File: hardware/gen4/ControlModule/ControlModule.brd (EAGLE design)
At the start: 29.9 x 59.3 mm, 39 parts, among them IC1 XMEGA16A4A

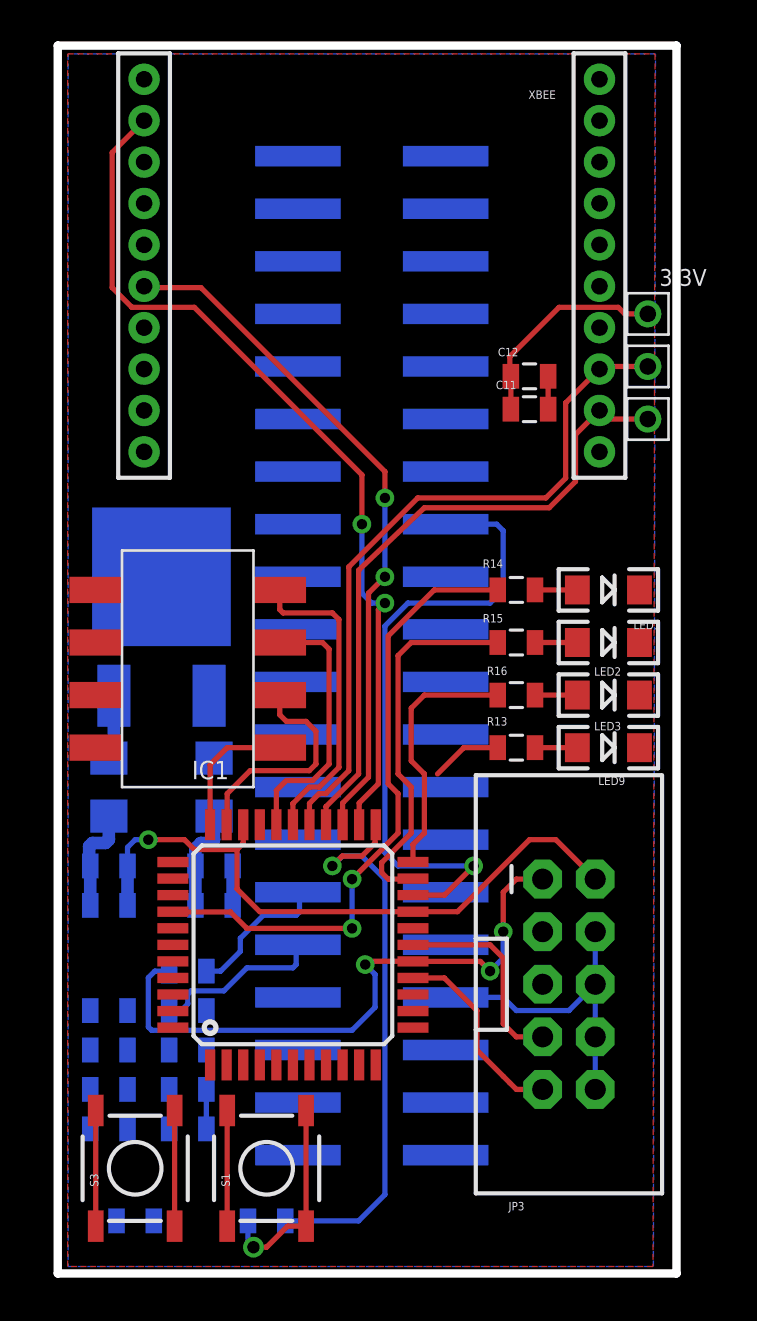
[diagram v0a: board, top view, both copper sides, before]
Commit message: routing fun!
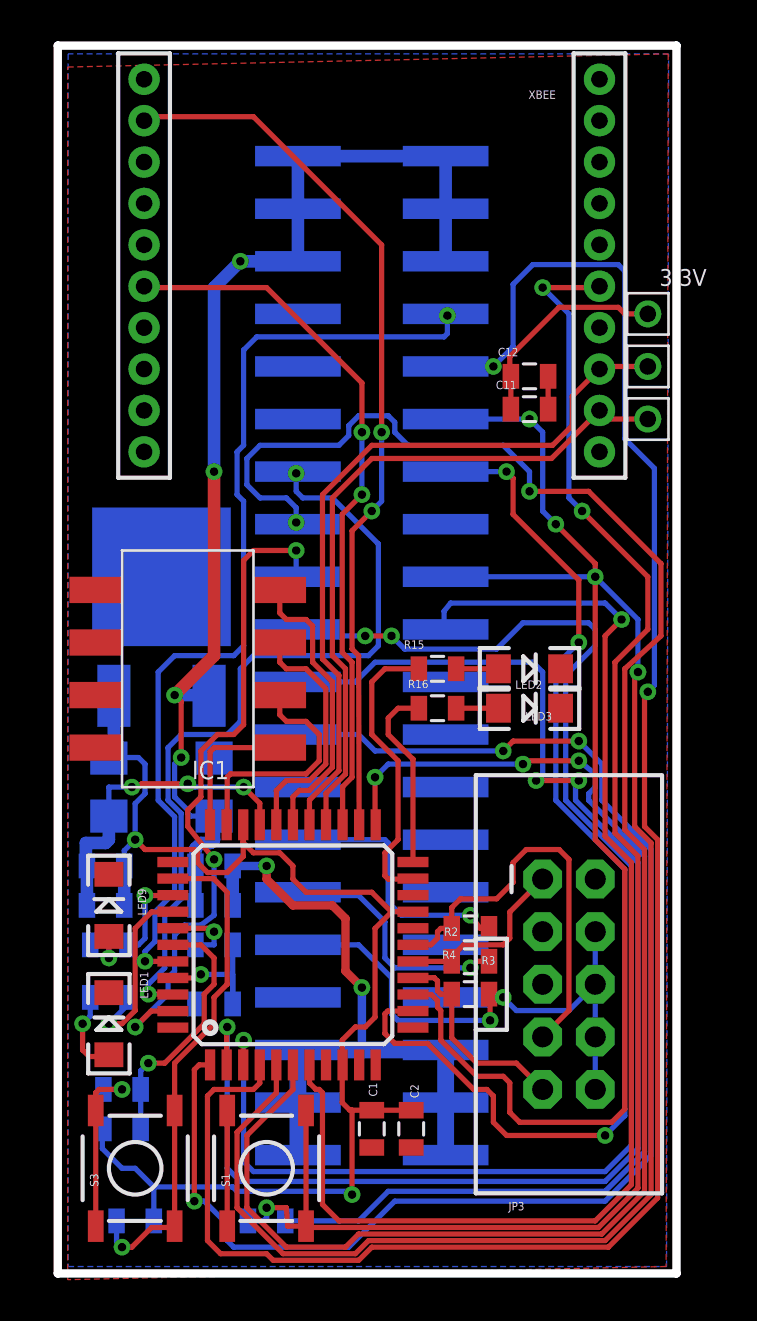
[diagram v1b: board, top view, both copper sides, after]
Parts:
- moved LED1 32.0 mm to (39.4, 19.1), turned to 90 degrees
- moved R14 27.8 mm to (39.4, 20.3), flipped to the bottom
- moved LED9 25.3 mm to (39.4, 24.8), turned to 90 degrees
- moved R13 21.9 mm to (39.4, 22.9), flipped to the bottom
- moved C2 15.7 mm to (54.0, 14.0), flipped to the top, turned to 270 degrees
- moved R4 14.9 mm to (56.8, 23.7), flipped to the top
- moved R3 13.7 mm to (56.8, 20.5), flipped to the top
- moved R2 13.7 mm to (56.8, 22.1), flipped to the top, turned to 0 degrees
- moved C1 13.3 mm to (52.1, 14.0), flipped to the top, turned to 270 degrees
- moved R9 7.10 mm to (44.5, 22.9)
- moved R8 6.16 mm to (44.5, 20.0)
- moved LED2 4.02 mm to (59.7, 36.2)
- moved R15 4.02 mm to (55.2, 36.2)
- moved LED3 3.86 mm to (59.7, 34.3)
- moved R16 3.86 mm to (55.2, 34.3)
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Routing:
- net BB_OUT: track 0.00 -> 92.5 mm, vias 0 -> 2
- net DISCHARGE: track 0.00 -> 90.3 mm, vias 0 -> 2
- net SS_1: track 0.00 -> 68.8 mm, vias 0 -> 3
- net SS_2: track 0.00 -> 68.4 mm, vias 0 -> 3
- net CHARGE_DONE: track 0.00 -> 68.1 mm, vias 0 -> 2
- net SS_3: track 0.00 -> 68.0 mm, vias 0 -> 3
- net XBRST: track 9.93 -> 76.1 mm, vias 1 -> 3
- net CHARGE: track 0.00 -> 61.2 mm, vias 0 -> 1
- net CHIP_ENABLE: track 0.00 -> 54.5 mm, vias 0 -> 3
- net KICK_ENABLE: track 0.00 -> 54.2 mm, vias 0 -> 2
- net 12V: track 4.97 -> 56.6 mm, vias 0 -> 4
- net BB_IN: track 0.00 -> 46.6 mm, vias 0 -> 2
- net DIVCAP: track 0.00 -> 38.6 mm, vias 0 -> 2
- net DRIB: track 0.00 -> 32.8 mm, vias 0 -> 3
- net KICK_REF: track 31.4 -> 0.00 mm, vias 1 -> 0
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
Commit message: routing comms board done
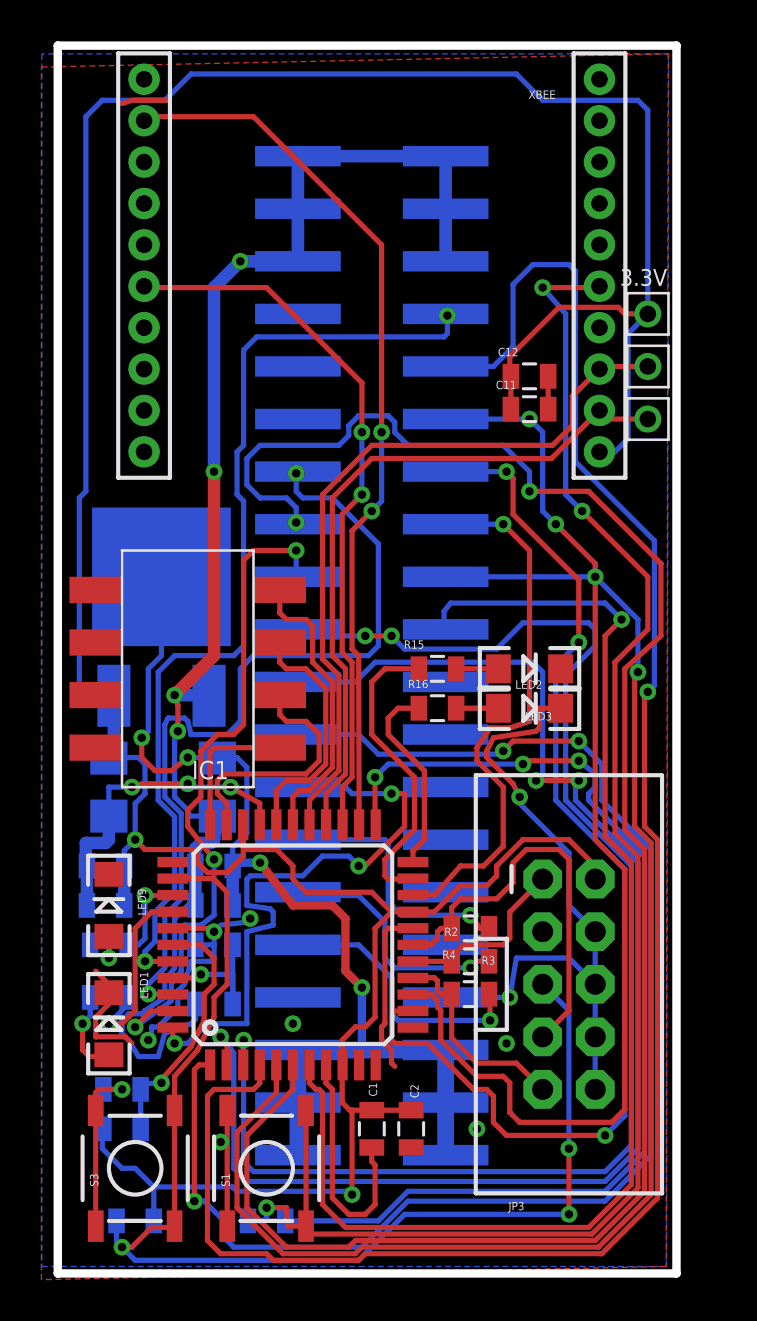
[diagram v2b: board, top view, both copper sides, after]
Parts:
- moved C4 0.16 mm to (44.6, 30.5)
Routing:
- net 3.3V: track 75.1 -> 163.2 mm
- net GND: track 50.6 -> 103.8 mm, vias 6 -> 13
- net RESET: track 24.4 -> 58.6 mm, vias 1 -> 3
- net SS_4: track 0.00 -> 29.6 mm, vias 0 -> 3
- net KICK_REF: track 0.00 -> 26.6 mm, vias 0 -> 1
- net 12VGND: track 32.8 -> 52.7 mm, vias 2 -> 4
- net 12V: track 56.6 -> 70.7 mm
- net DIVCAP: track 38.6 -> 40.5 mm
- net BB_OUT: track 92.5 -> 91.1 mm, vias 2 -> 1
- net SS_2: track 68.4 -> 67.5 mm
- net GLED2: track 14.1 -> 14.8 mm
- net BID2: track 11.6 -> 12.2 mm
